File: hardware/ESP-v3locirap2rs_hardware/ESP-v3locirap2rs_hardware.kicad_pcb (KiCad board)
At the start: 2 copper layers, 2 parts, among them U1 ESP32-DEVKITC-32D

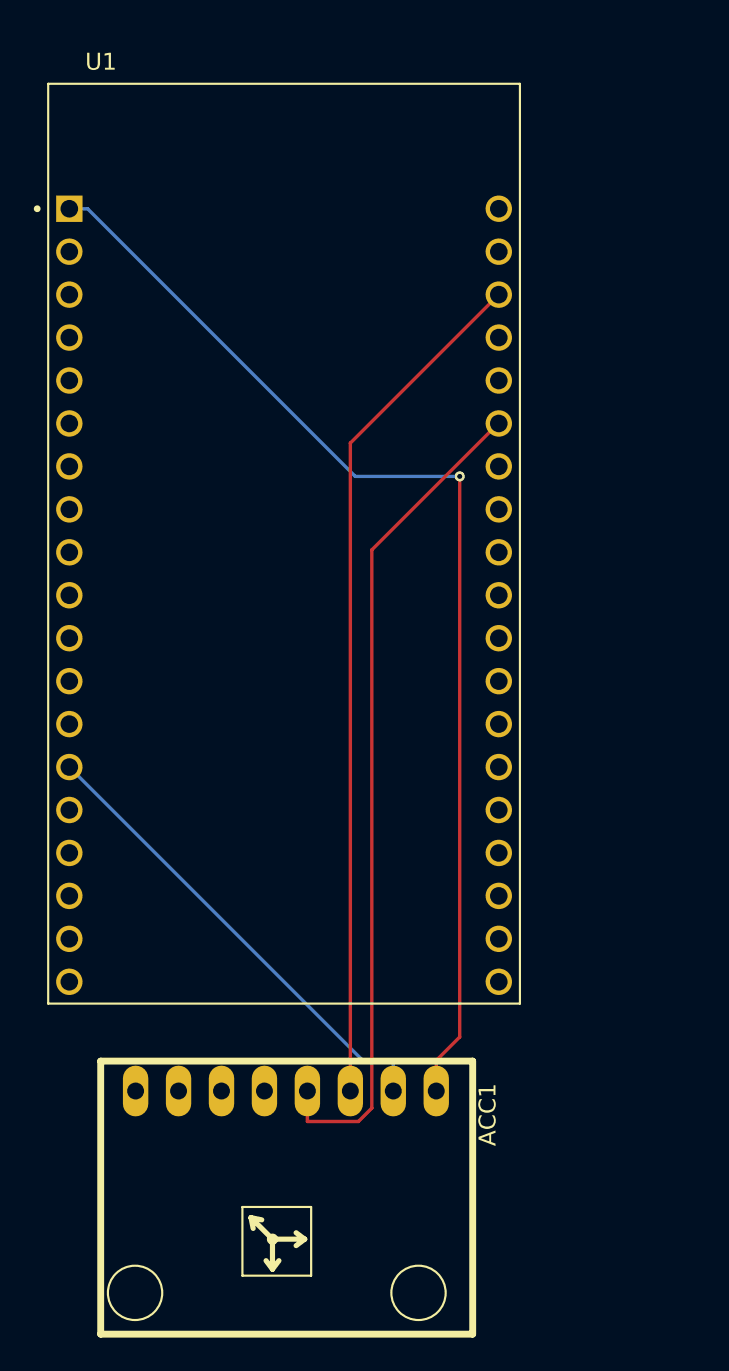
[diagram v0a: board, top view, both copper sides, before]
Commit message: kicad pcb updates
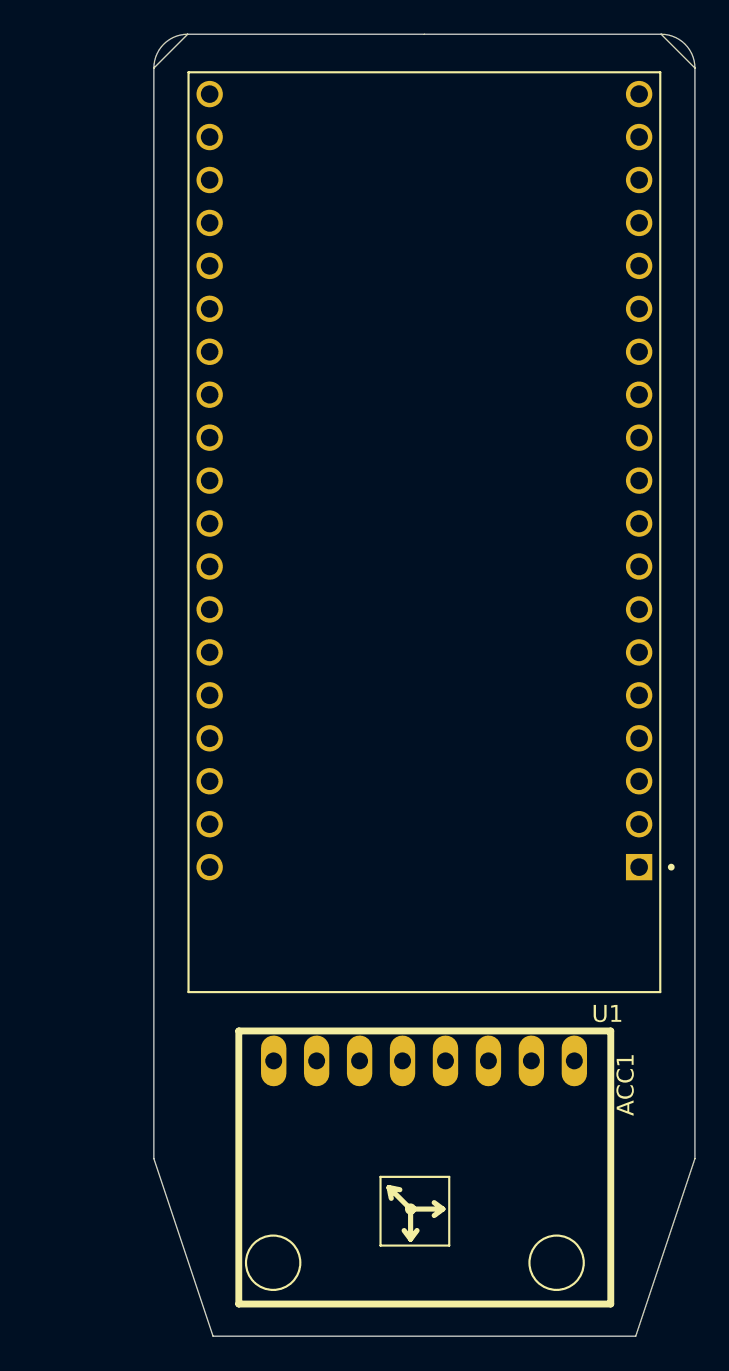
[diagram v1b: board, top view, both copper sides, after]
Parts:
- moved ACC1 8.36 mm to (101.5, 111.4)
- moved U1 8.32 mm to (112.5, 82.0), turned to 180 degrees
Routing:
- net /ESP32/3.3V: track 66.6 -> 0.00 mm, vias 1 -> 0
- net /ESP32/SCL: track 50.7 -> 0.00 mm
- net /ESP32/SDA: track 49.6 -> 0.00 mm
- net GND: track 28.2 -> 0.00 mm
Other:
- board outline added: 32 x 77 mm
